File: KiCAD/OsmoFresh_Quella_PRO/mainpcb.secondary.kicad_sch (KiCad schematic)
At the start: 7 parts, among them K2 [NO]

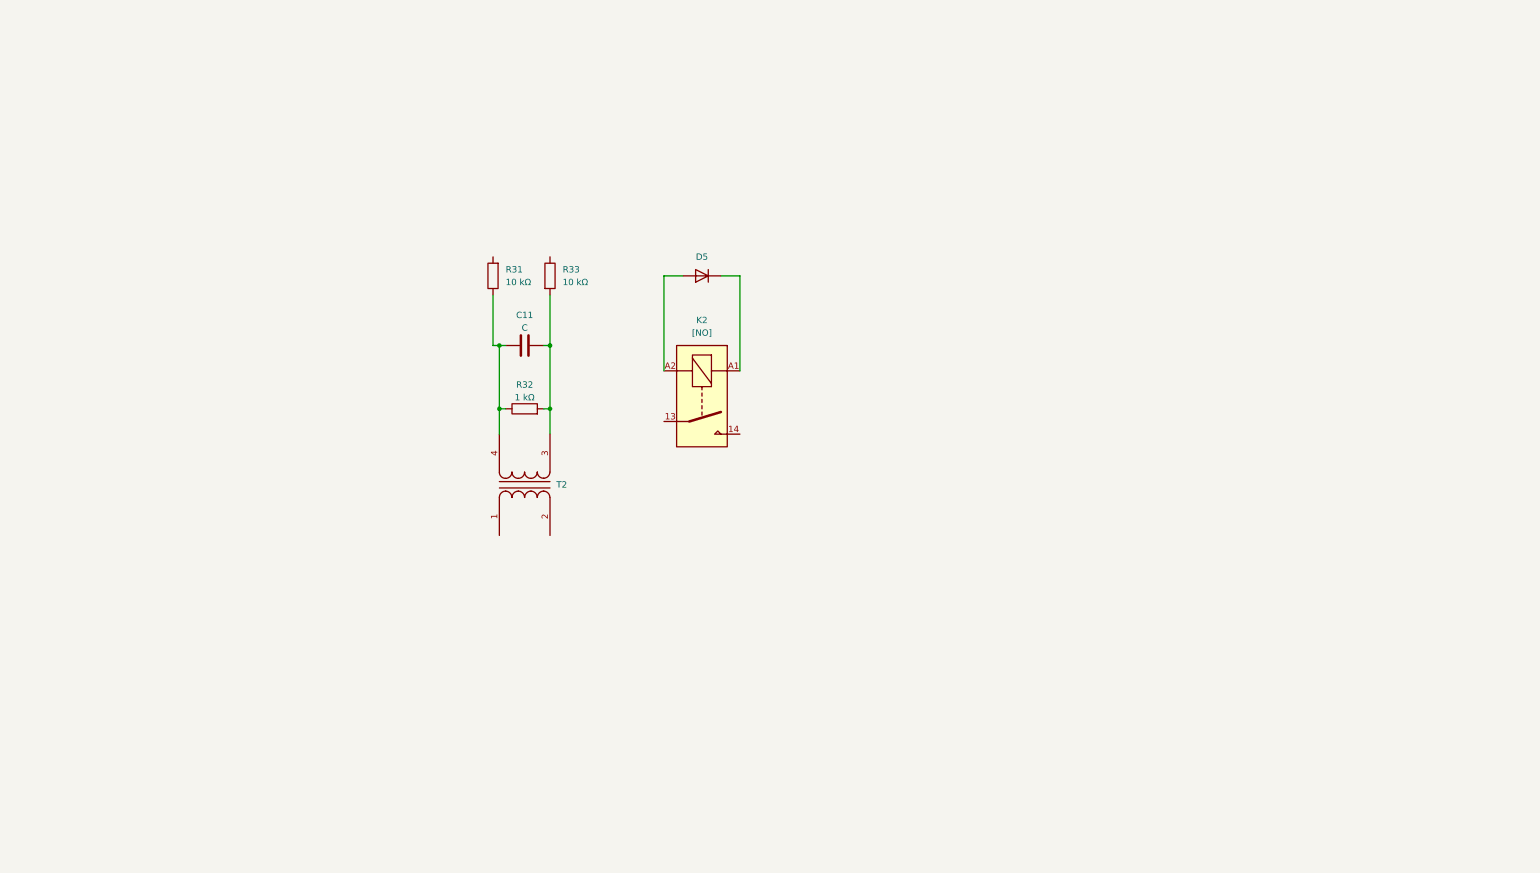
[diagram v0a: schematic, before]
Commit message: Update Schematics
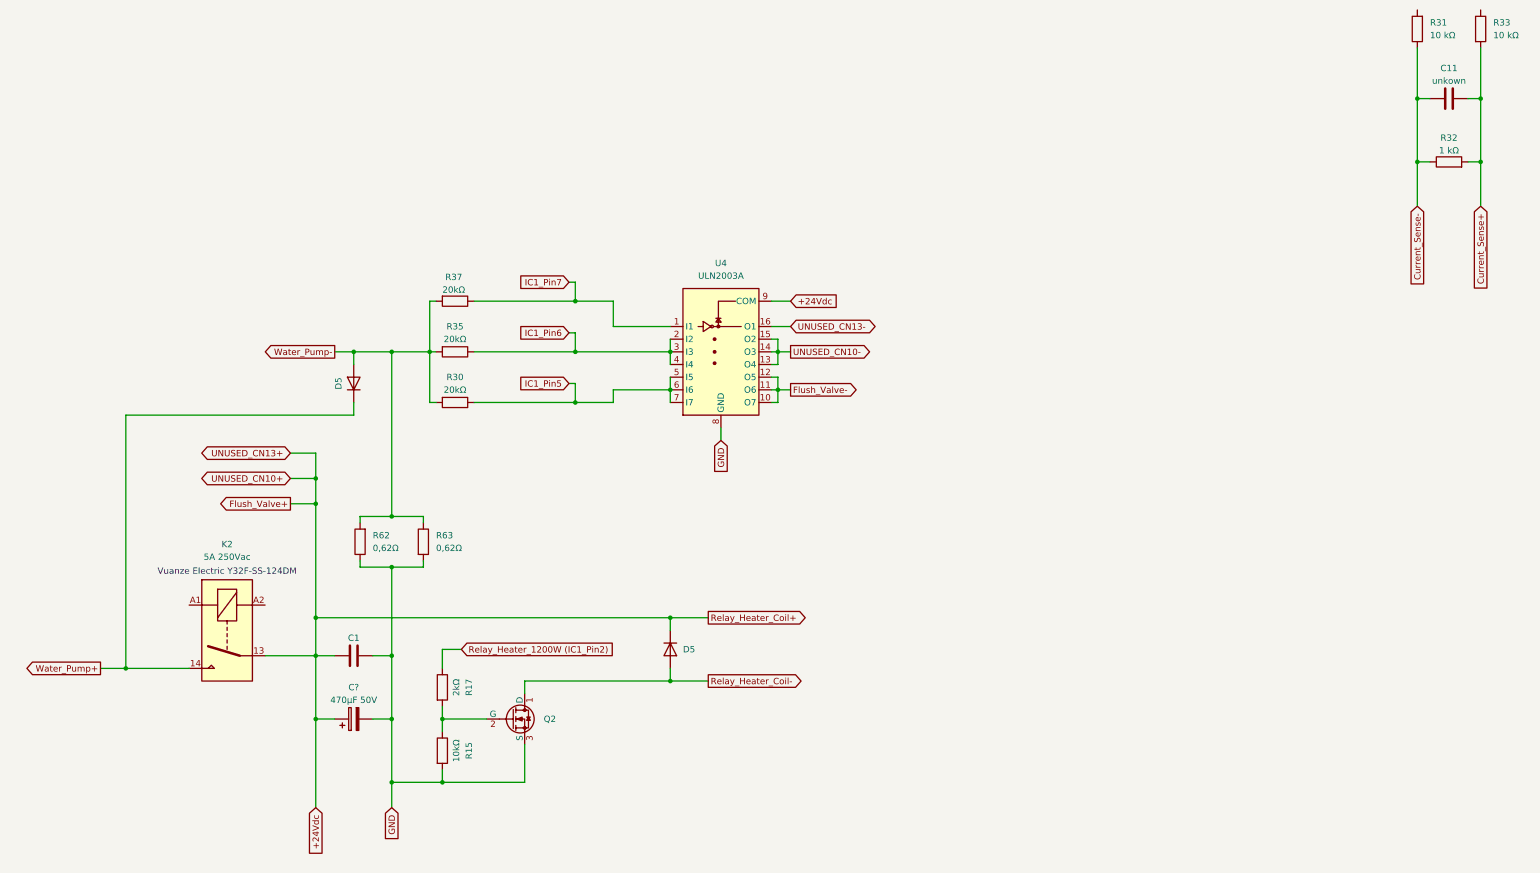
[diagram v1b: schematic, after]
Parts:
- removed T2: (no value), symbol Device:Transformer_1P_1S
- added C1: (no value), symbol Device:C
- added C?: 470µF 50V, symbol Device:C_Polarized
- added D5: D, symbol Device:D
- added Q2: (no value), symbol Transistor_FET:Q_NMOS_DGS
- added R15: 10kΩ, symbol Device:R
- added R17: 2kΩ, symbol Device:R
- added R30, R35, R37: 20kΩ, symbol Device:R
- added R62, R63: 0,62Ω, symbol Device:R
- added U4: ULN2003A, symbol Transistor_Array:ULN2003A
- C11: value C -> unkown
- K2: value [NO] -> 5A 250Vac
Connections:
- net Current_Sense+: now reaches C11.2, R32.2, R33.2
- net at K2.A1: no longer D5.1 (K)
- net at K2.A2: no longer D5.2 (A)
- net Current_Sense-: now reaches C11.1, R31.1, R32.1
- net +24Vdc: now reaches K2.13
- net +24Vdc: now also D5.1 (K), C1.1, C?.1, U4.9 (COM)
- net Water_Pump+: now reaches K2.14
- net Water_Pump+: now also D5.1 (K)
- new net: Q2.2 (G), R15.1, R17.2
- new net Flush_Valve-: U4.10 (O7), U4.11 (O6), U4.12 (O5)
- new net GND: C1.2, C?.2, Q2.3 (S), R15.2, R62.1, R63.2, U4.8 (GND)
- new net IC1_Pin5: R30.1, U4.5 (I5), U4.6 (I6), U4.7 (I7)
- new net IC1_Pin6: R35.1, U4.2 (I2), U4.3 (I3), U4.4 (I4)
- new net IC1_Pin7: R37.1, U4.1 (I1)
- new net Relay_Heater_1200W (IC1_Pin2): R17.1
- new net Relay_Heater_Coil-: D5.2 (A), Q2.1 (D)
- new net UNUSED_CN10-: U4.13 (O4), U4.14 (O3), U4.15 (O2)
- new net UNUSED_CN13-: U4.16 (O1)
- new net Water_Pump-: D5.2 (A), R30.2, R35.2, R37.2, R62.2, R63.1
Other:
- note added: "Vuanze Electric Y32F-SS-124DM"
- title: MainPCB.Secondary -> MainPCB Secondary
- moved on the sheet: C11, D5, R31, R32, R33

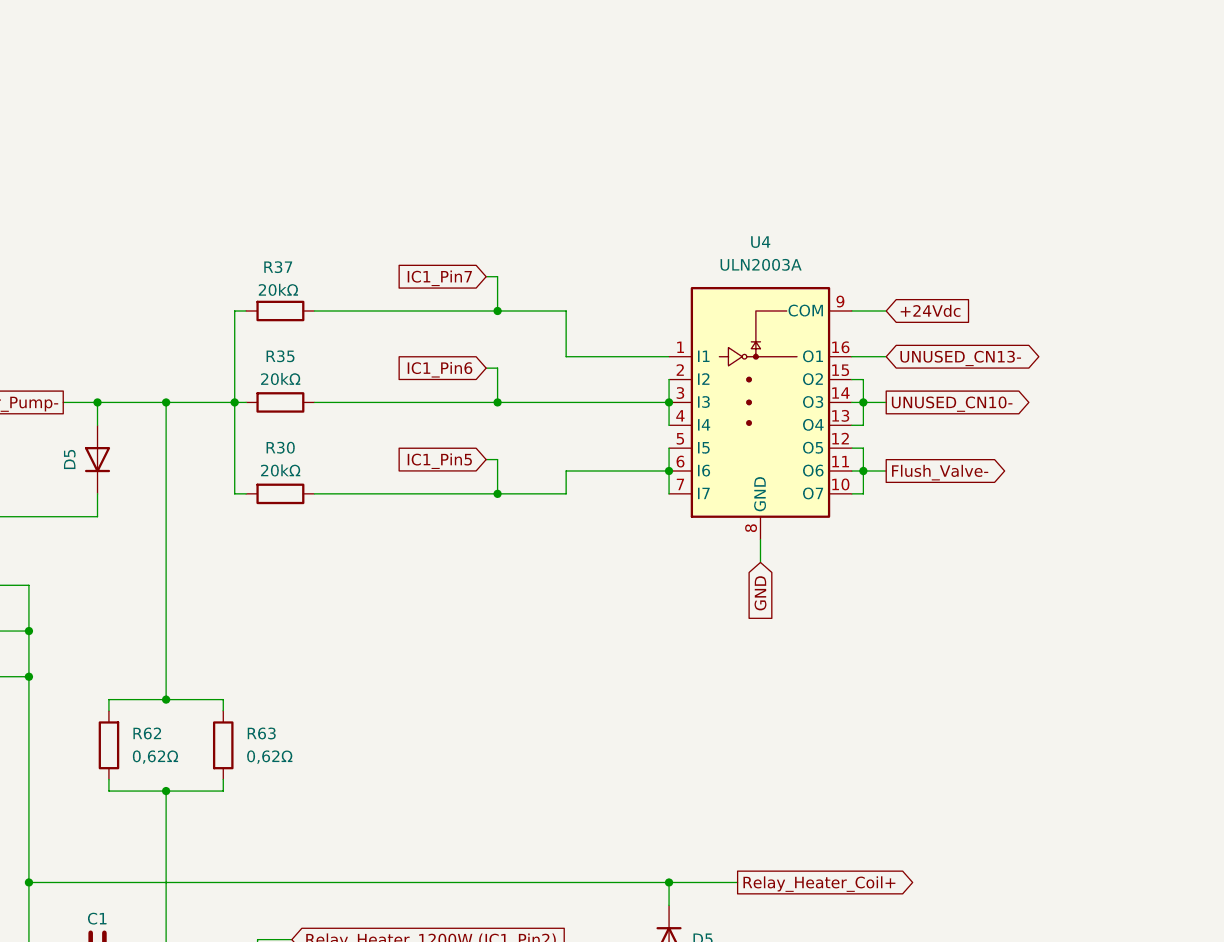
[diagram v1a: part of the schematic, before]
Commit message: Update Filestructure
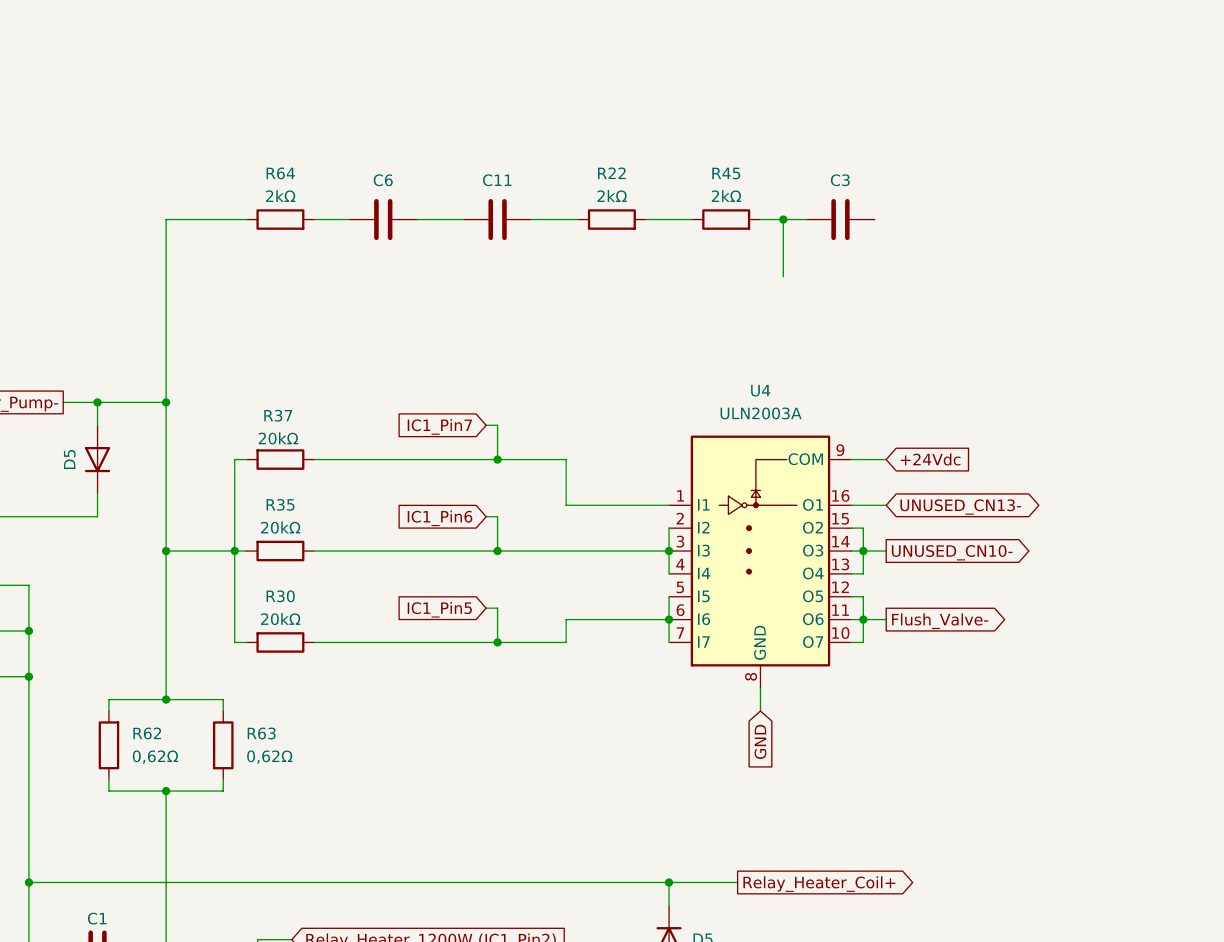
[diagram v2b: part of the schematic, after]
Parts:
- added C11, C3, C6: C, symbol Device:C
- added R22, R45, R64: 2kΩ, symbol Device:R
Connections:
- net Water_Pump-: now also R64.1
- new net: C3.1, R45.2
- new net: C6.1, R64.2
- new net: C11.1, C6.2
- new net: C11.2, R22.1
- new net: R22.2, R45.1
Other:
- moved on the sheet: R30, R35, R37, U4
